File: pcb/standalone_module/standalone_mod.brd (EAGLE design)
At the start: 31 x 31.2 mm, 11 parts, among them U1 V_REG_317DPACK

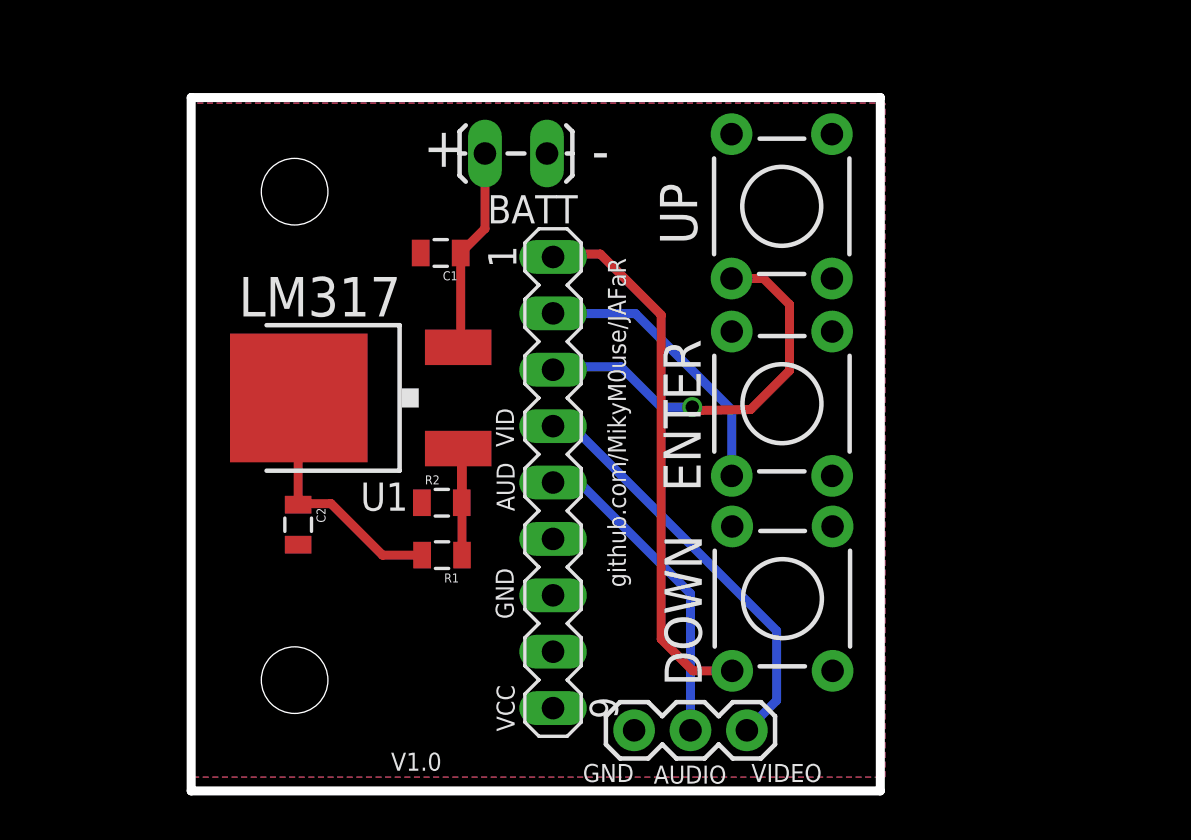
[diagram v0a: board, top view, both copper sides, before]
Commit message: standalone v2.0
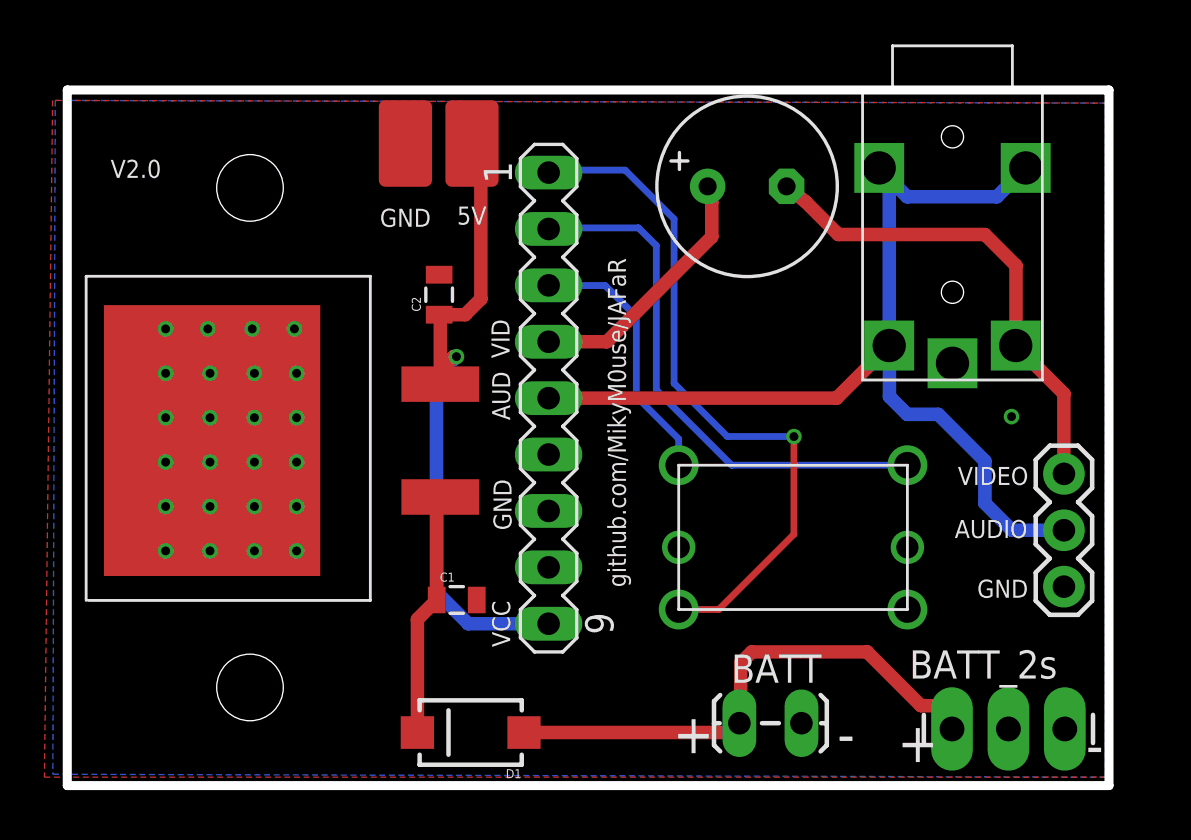
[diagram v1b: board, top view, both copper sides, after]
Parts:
- removed R1, R2: (no value), SparkFun-Passives:0805
- removed S1, S2, S3: SWITCH-MOMENTARY-2PTH, SparkFun-Electromechanical:TACTILE-PTH
- removed U1: V_REG_317DPACK, SparkFun-PowerIC:V-REG_DPACK
- added C3: (no value), resistor:E3,5-8
- added D1: (no value), SparkFun-DiscreteSemi:SMA-DIODE
- added JP3: (no value), SparkFun-Connectors:1X03_LONGPADS
- added JP4, JP5: (no value), SparkFun-Connectors:LUXEON-PAD
- added U$1: 7805, #fpv:DDPAK
- added U$2: SKQUCAA010, #fpv:SKQUCAA010
- added U$3: MC001293JACK, #fpv:MC001293
- C1: value (none) -> 0.33uF
- C2: value (none) -> 0.1uF
- moved BATT 28.1 mm to (27.7, 3.39)
- moved JP2 20.4 mm to (39.7, 9.54), turned to 90 degrees
- moved C1 15.6 mm to (12.3, 8.94), turned to 0 degrees
- moved C2 12.2 mm to (11.5, 22.7), turned to 90 degrees
- moved JP1 3.81 mm to (16.4, 18.0)
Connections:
- removed net 3.3V: C2.1, R1.2, U1.4
- removed net N$4: R1.1, R2.2, U1.1
- new net N$2: C3.+, JP1.4
- new net N$3: BATT.2, D1.A, JP3.3
- net 5V: now also C2.1, JP4.P$1, U$1.OUTPUT
- net AUDOUT: now also U$3.3_1, U$3.3_2, U$3.4
- net DOWN: now also U$2.3; no longer S1.1
- net ENTER: now also U$2.6; no longer S2.1
- net GND: now also JP3.1, JP5.P$1, U$1.GND, U$2.4, U$3.1; no longer R2.1, S1.3, S2.3, S3.3
- net N$1: now also D1.C, U$1.INPUT; no longer BATT.2, U1.3
- net UP: now also U$2.1; no longer S3.1
- net VIDOUT: now also C3.-, U$3.2; no longer JP1.4
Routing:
- net AUDOUT: track 14.4 -> 46.0 mm
- net 5V: track 0.00 -> 30.0 mm, vias 0 -> 1
- net N$3: track 0.00 -> 24.7 mm
- net N$2: track 0.00 -> 11.6 mm
- net ENTER: track 12.8 -> 24.4 mm
- net 3.3V: track 11.4 -> 0.00 mm
- net N$4: track 7.38 -> 0.00 mm
- net DOWN: track 24.5 -> 31.4 mm, vias 0 -> 1
- net UP: track 18.3 -> 12.0 mm, vias 1 -> 0
- net VIDOUT: track 18.9 -> 22.1 mm
- net N$1: track 9.30 -> 11.0 mm
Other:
- board size 31 x 31.2 mm -> 46.9 x 31.3 mm
- board text added: "5V"
- board text added: "BATT_2s"
- board text added: "V2.0"
- board text removed: "DOWN"
- board text removed: "ENTER"
- board text removed: "LM317"
- board text removed: "UP"
- board text removed: "V1.0"
